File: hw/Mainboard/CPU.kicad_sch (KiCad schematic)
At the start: 8 parts, among them U11 W65C02S, U12 AS6C1008

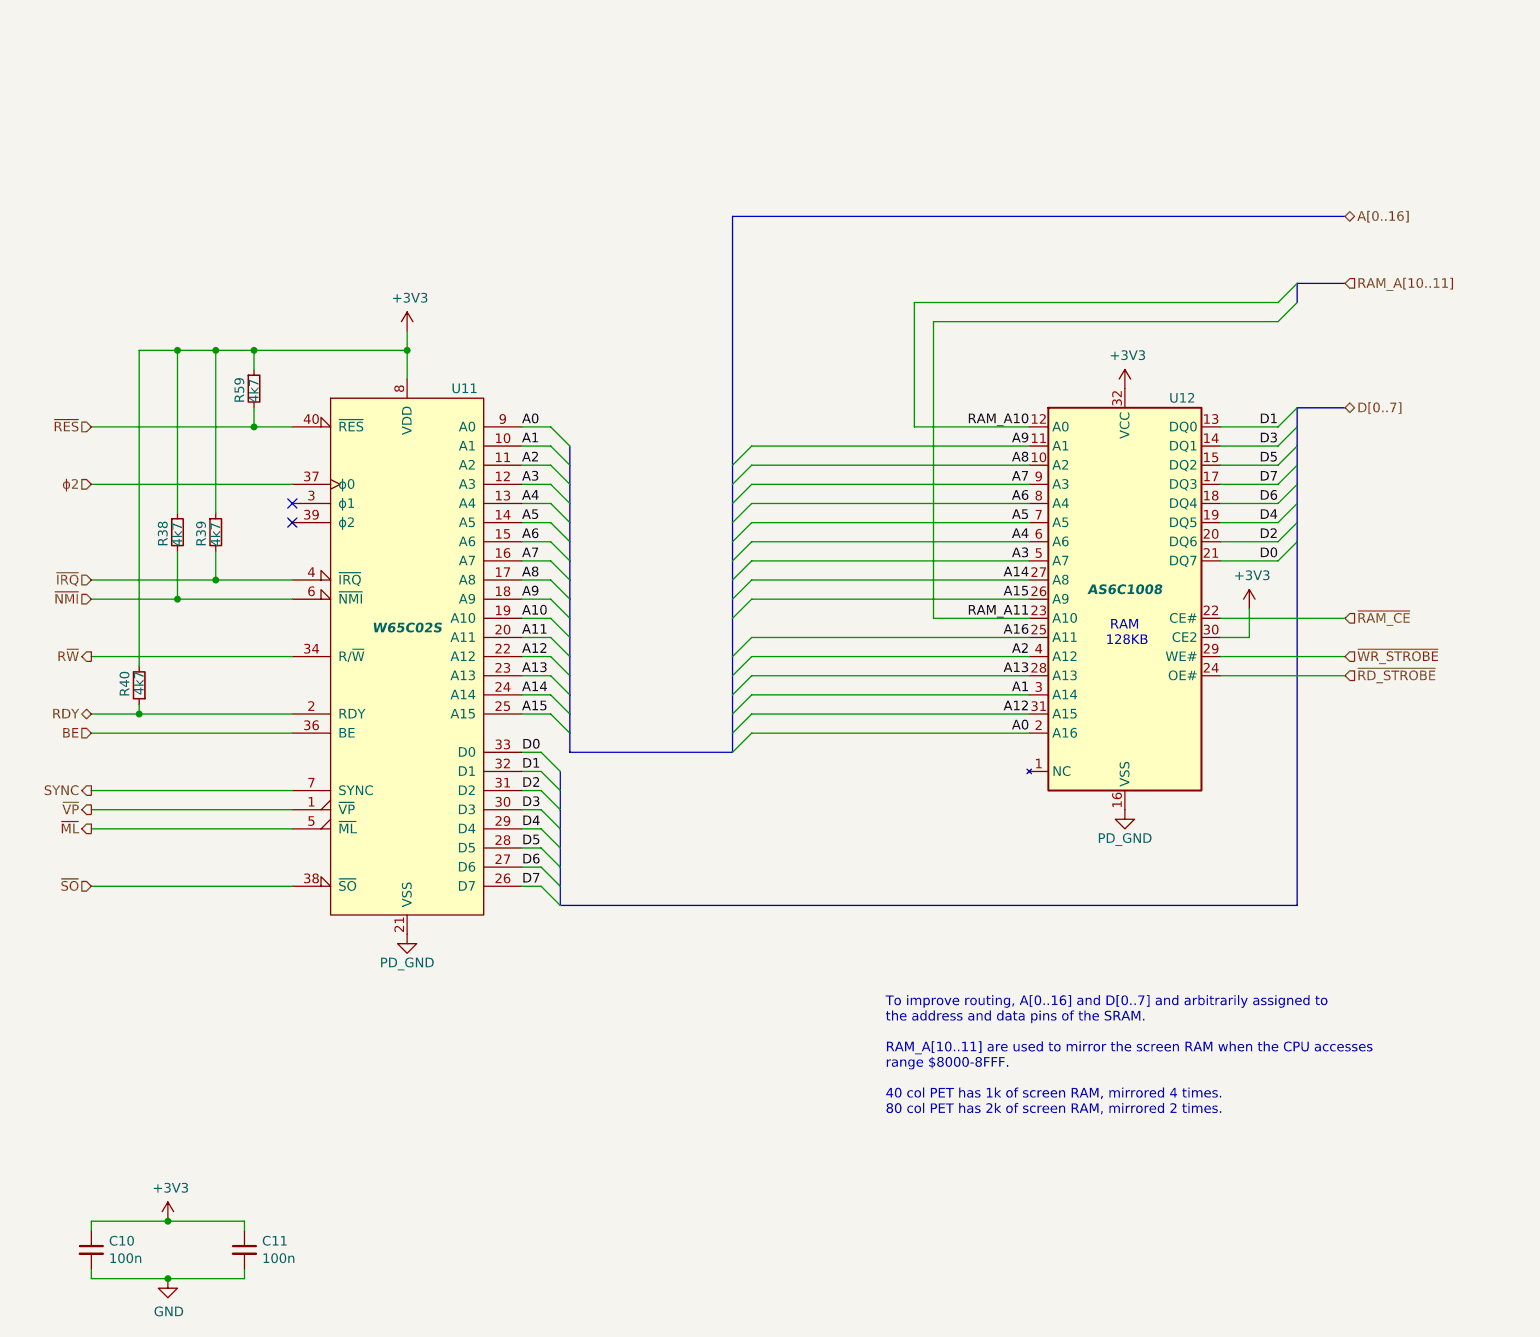
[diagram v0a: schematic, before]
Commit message: hw: wip
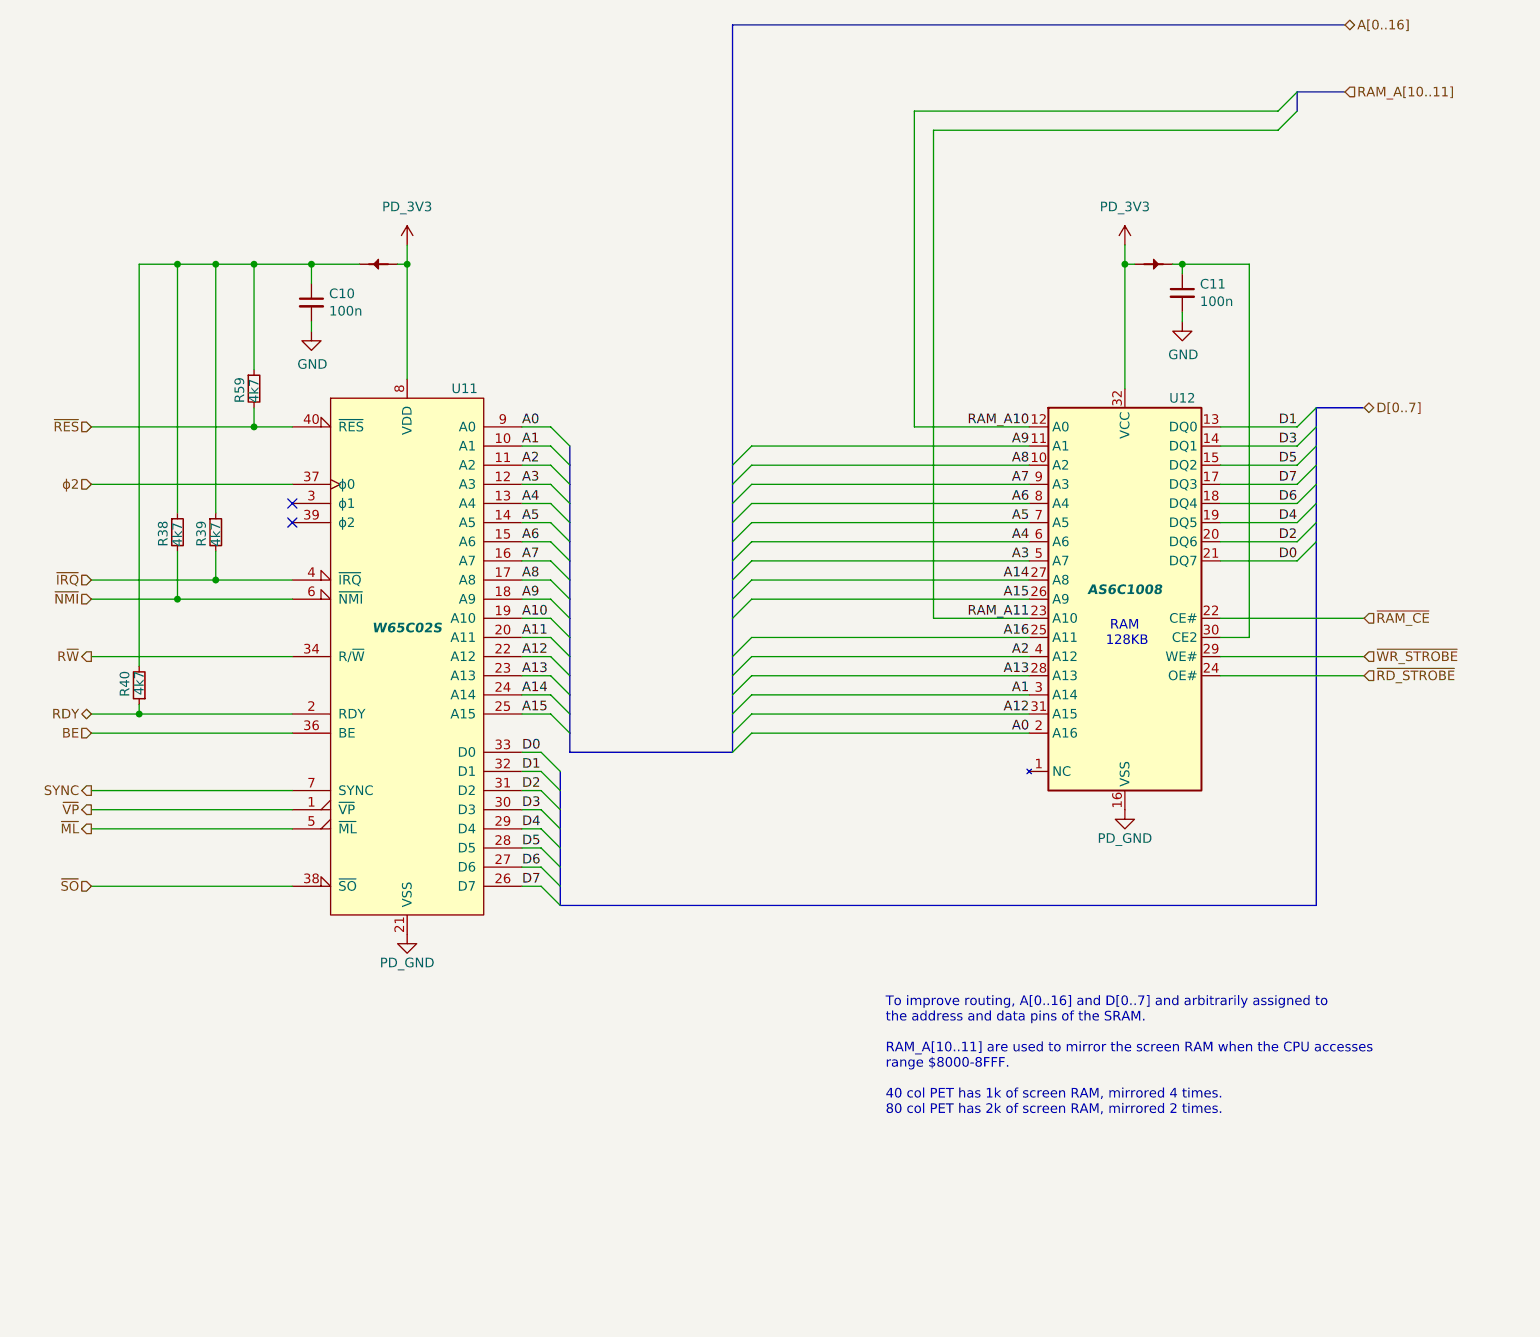
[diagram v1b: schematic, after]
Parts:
- added PT1, PT2: PowerTie_2, PET:NetTie-2_SMD_Pad_1.6_to_0.4mm, symbol PET:PowerTie_2
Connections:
- net +3V3: no longer names the net of C10.1, R38.1, R39.1, R40.2, R59.1
- net +3V3: now also PT1.2; no longer C11.1, U11.8 (VDD), U12.30 (CE2), U12.32 (VCC)
- new net: C11.1, PT2.2, U12.30 (CE2)
- new net PD_3V3: PT1.1, PT2.1, U11.8 (VDD), U12.32 (VCC)
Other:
- moved on the sheet: C10, C11
